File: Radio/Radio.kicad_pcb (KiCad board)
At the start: 2 copper layers, 56.6 x 68.7 mm, 36 parts, among them IC1 SI4844-A10-GU, J1 AudioJack3, J2 Conn_01x04_Pin, J3 Conn_01x02_Socket, J4 Conn_01x07_Pin, Q1 NPN, U1 ARDUINO_PRO_MINI, Y1 32.768 kHz

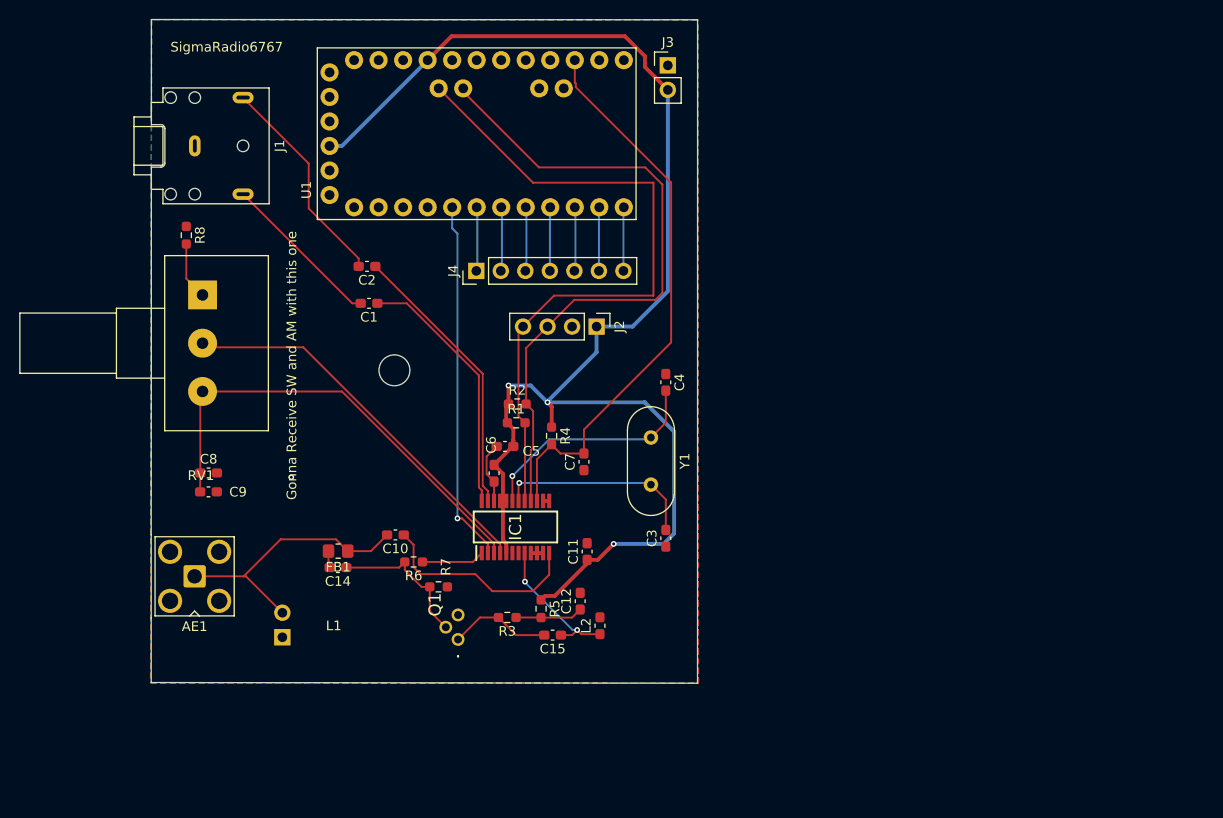
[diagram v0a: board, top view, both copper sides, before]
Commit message: Updated PCB
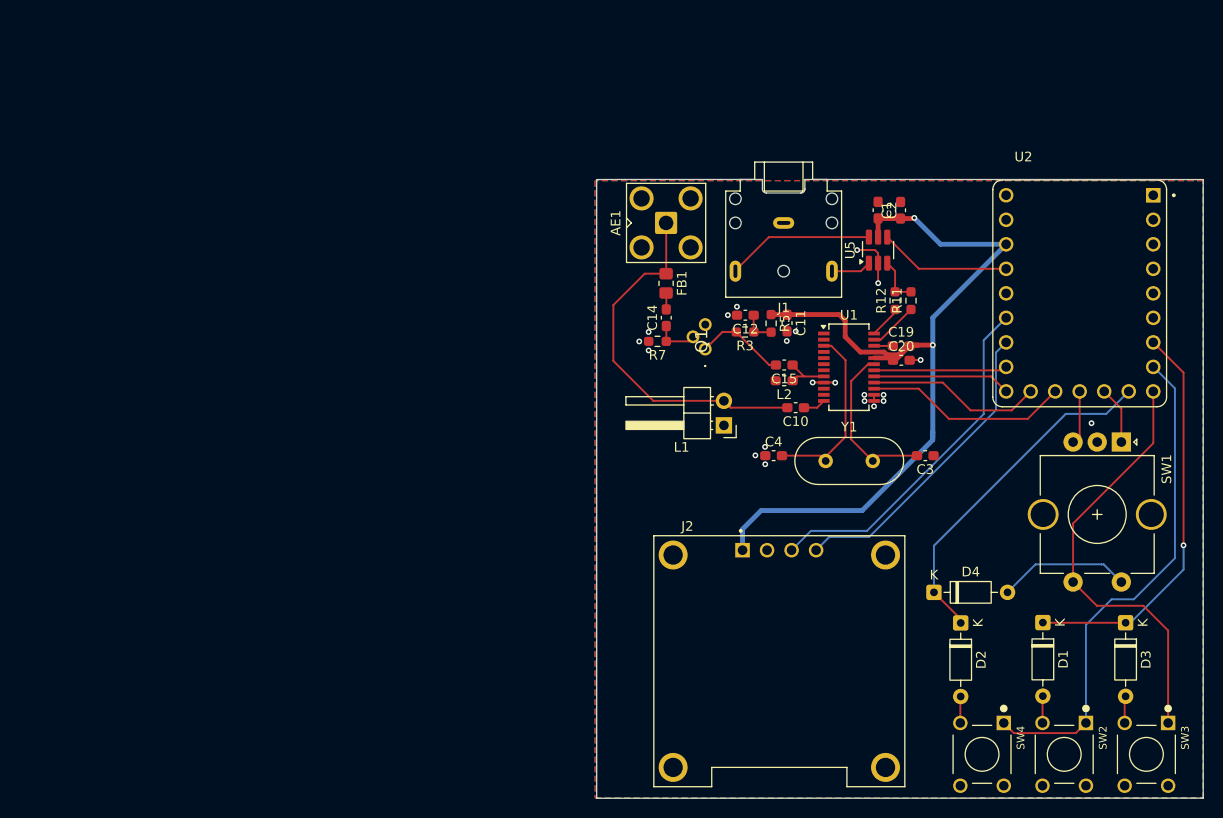
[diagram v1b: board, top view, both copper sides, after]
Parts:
- removed C5: 4.7uF, Capacitor_SMD:C_0603_1608Metric_Pad1.08x0.95mm_HandSolder
- removed C6, C7, C9: 0.1uF, Capacitor_SMD:C_0603_1608Metric_Pad1.08x0.95mm_HandSolder
- removed C8: 47uF, Capacitor_SMD:C_0603_1608Metric_Pad1.08x0.95mm_HandSolder
- removed IC1: SI4844-A10-GU, RadioLib:SOP64P600X175-24N
- removed J3: Conn_01x02_Socket, Connector_PinHeader_2.54mm:PinHeader_1x02_P2.54mm_Vertical
- removed J4: Conn_01x07_Pin, Connector_PinHeader_2.54mm:PinHeader_1x07_P2.54mm_Vertical
- removed R1, R2: 2.2K, Resistor_SMD:R_0603_1608Metric_Pad0.98x0.95mm_HandSolder
- removed R4: 100K, Resistor_SMD:R_0603_1608Metric_Pad0.98x0.95mm_HandSolder
- removed R6: 120K, Resistor_SMD:R_0603_1608Metric_Pad0.98x0.95mm_HandSolder
- removed R8: 100, Resistor_SMD:R_0603_1608Metric_Pad0.98x0.95mm_HandSolder
- removed REF**: MountingHole_3.2mm_M3_DIN965, MountingHole:MountingHole_3.2mm_M3_DIN965
- removed RV1: 100K, Potentiometer_THT:Potentiometer_Alps_RK163_Single_Horizontal
- added C19: 22nF, Capacitor_SMD:C_0603_1608Metric_Pad1.08x0.95mm_HandSolder, F.Cu at (148.7, 50.5)
- added C20: 100nF, Capacitor_SMD:C_0603_1608Metric_Pad1.08x0.95mm_HandSolder, F.Cu at (148.8, 52.0)
- added D1: 1N4148, Diode_THT:D_DO-35_SOD27_P7.62mm_Horizontal, F.Cu at (163.4, 79.2)
- added D2: 1N4148, Diode_THT:D_DO-35_SOD27_P7.62mm_Horizontal, F.Cu at (154.9, 79.2)
- added D3: 1N4148, Diode_THT:D_DO-35_SOD27_P7.62mm_Horizontal, F.Cu at (172.0, 79.2)
- added D4: 1N4148, Diode_THT:D_DO-35_SOD27_P7.62mm_Horizontal, F.Cu at (152.1, 76.1)
- added R11: 1k, Resistor_SMD:R_0603_1608Metric_Pad0.98x0.95mm_HandSolder, F.Cu at (149.8, 45.9)
- added R12: 1k, Resistor_SMD:R_0603_1608Metric_Pad0.98x0.95mm_HandSolder, F.Cu at (148.1, 45.9)
- added SW1: RotaryEncoder_Switch, Rotary_Encoder:RotaryEncoder_Alps_EC11E-Switch_Vertical_H20mm_CircularMountingHoles, F.Cu at (171.6, 60.5)
- added SW2: SW_Push_45deg, FSM8JH:SW_FSM8JH, F.Cu at (165.6, 92.9)
- added SW3: SW_Push_45deg, FSM8JH:SW_FSM8JH, F.Cu at (174.1, 92.9)
- added SW4: SW_Push_45deg, FSM8JH:SW_FSM8JH, F.Cu at (157.1, 92.9)
- added U2: RP2040-ZERO, RP2040-ZERO:MODULE_RP2040-ZERO, F.Cu at (167.2, 45.1)
- added U5: PAM8301, Package_TO_SOT_SMD:SOT-23-6_Handsoldering, F.Cu at (146.3, 40.6)
- C1: value 4.7uF -> 10uF
- C2: value 4.7uF -> 0.1uF
- J2: footprint Connector_PinHeader_2.54mm:PinHeader_1x04_P2.54mm_Vertical -> DM-OLED096-636:MODULE_DM-OLED096-636
- L1: moved to F.Cu
- U1: value ARDUINO_PRO_MINI -> Si4735-D60-GU; footprint ARDUINO_PRO_MINI:MODULE_ARDUINO_PRO_MINI -> Package_SO:SSOP-24_3.9x8.7mm_P0.635mm
- moved J1 61.5 mm to (136.6, 37.8), turned to 180 degrees
- moved AE1 61.0 mm to (124.4, 37.8), turned to 0 degrees
- moved C1 55.9 mm to (148.7, 36.5), turned to 90 degrees
- moved C2 53.3 mm to (146.3, 36.5), turned to -90 degrees
- moved L1 50.7 mm to (130.4, 58.8), turned to 180 degrees
- moved U1 45.5 mm to (143.3, 52.8), turned to 0 degrees
- moved FB1 43.9 mm to (124.4, 44.1), turned to -90 degrees
- moved C10 43.5 mm to (137.8, 57.0)
- moved C14 42.7 mm to (124.4, 47.6), turned to 90 degrees
- moved Q1 39.5 mm to (128.4, 50.9)
- moved J2 39.5 mm to (136.1, 83.2), turned to 0 degrees
- moved R3 38.5 mm to (132.6, 49.1)
- moved R5 38.0 mm to (135.3, 48.2)
- moved C15 36.9 mm to (136.6, 52.5)
- moved C12 34.2 mm to (132.6, 47.4), turned to 180 degrees
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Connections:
- C1 pad 1: Net-(IC1-LOUT) -> +3V3
- C1 pad 2: Net-(C1-Pad2) -> GND
- C10 pad 1: Net-(IC1-AMI) -> AM_ANT_IC
- C2 pad 1: Net-(IC1-ROUT) -> GND
- C2 pad 2: Net-(C2-Pad2) -> +3V3
- J1 pad R: Net-(C2-Pad2) -> Net-(U5-OUT-)
- J1 pad T: Net-(C1-Pad2) -> Net-(U5-OUT+)
- J2 pad 3: SDIO -> SDA_OLED
- J2 pad 4: SCLK -> SCLK_OLED
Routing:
- net SDIO: track 68.9 -> 0.00 mm
- net +3V3: track 152.2 -> 91.7 mm, vias 3 -> 2
- net SCLK: track 71.5 -> 14.3 mm
- net TUNE1: track 48.2 -> 0.00 mm
- net ROW1: track 6.66 -> 52.4 mm
- net TUNE2: track 40.5 -> 0.00 mm
- net ROW2: track 6.50 -> 44.7 mm
- net IRQ: track 37.6 -> 0.00 mm, vias 1 -> 0
- net RST: track 58.8 -> 21.2 mm
- net SDA_OLED: track 0.00 -> 36.7 mm
- net COL1: track 6.66 -> 41.7 mm, vias 0 -> 1
- net SCLK_OLED: track 0.00 -> 32.1 mm
- net COL2: track 6.66 -> 35.9 mm
- net Net-(IC1-ROUT): track 29.1 -> 0.00 mm
- net Net-(IC1-LOUT): track 26.9 -> 0.00 mm
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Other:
- board size 56.6 x 68.7 mm -> 62.8 x 64.1 mm
- board text removed: "Gonna Receive SW and AM with this one"
- board text removed: "SigmaRadio6767"
